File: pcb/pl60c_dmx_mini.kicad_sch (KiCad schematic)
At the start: 35 parts, among them J1 USB-C 16P, J2 XLR-5 female (DMX OUT), Q1 S8050, SW2 BOOT, SW3 USER, U1 ESP32-S3-MINI-1-N8, U2 AP2112K-3.3, U3 SP3485EN, U4 USBLC6-2SC6

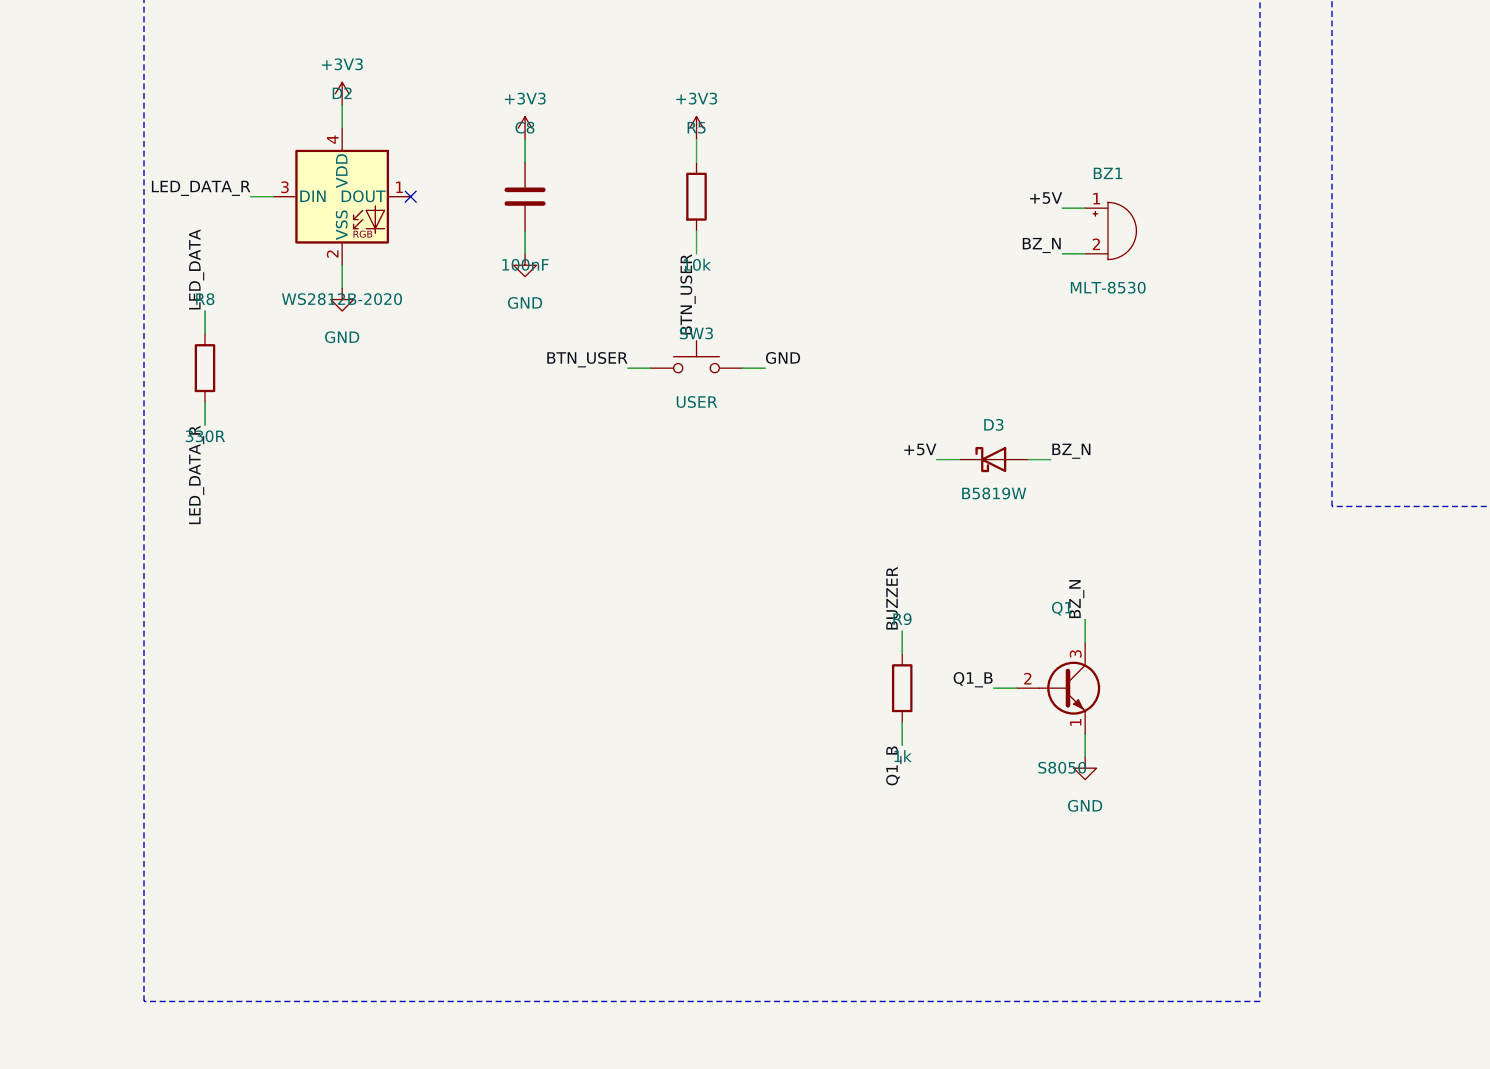
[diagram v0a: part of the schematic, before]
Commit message: auto: 2026-09-02 14:14:01
Co-Authored-By: Claude Fable 5.1 <noreply@anthropic.com>
Claude-Session: https://claude.ai/code/session_01WsrVZb94LwbHVAmBvsSTfn
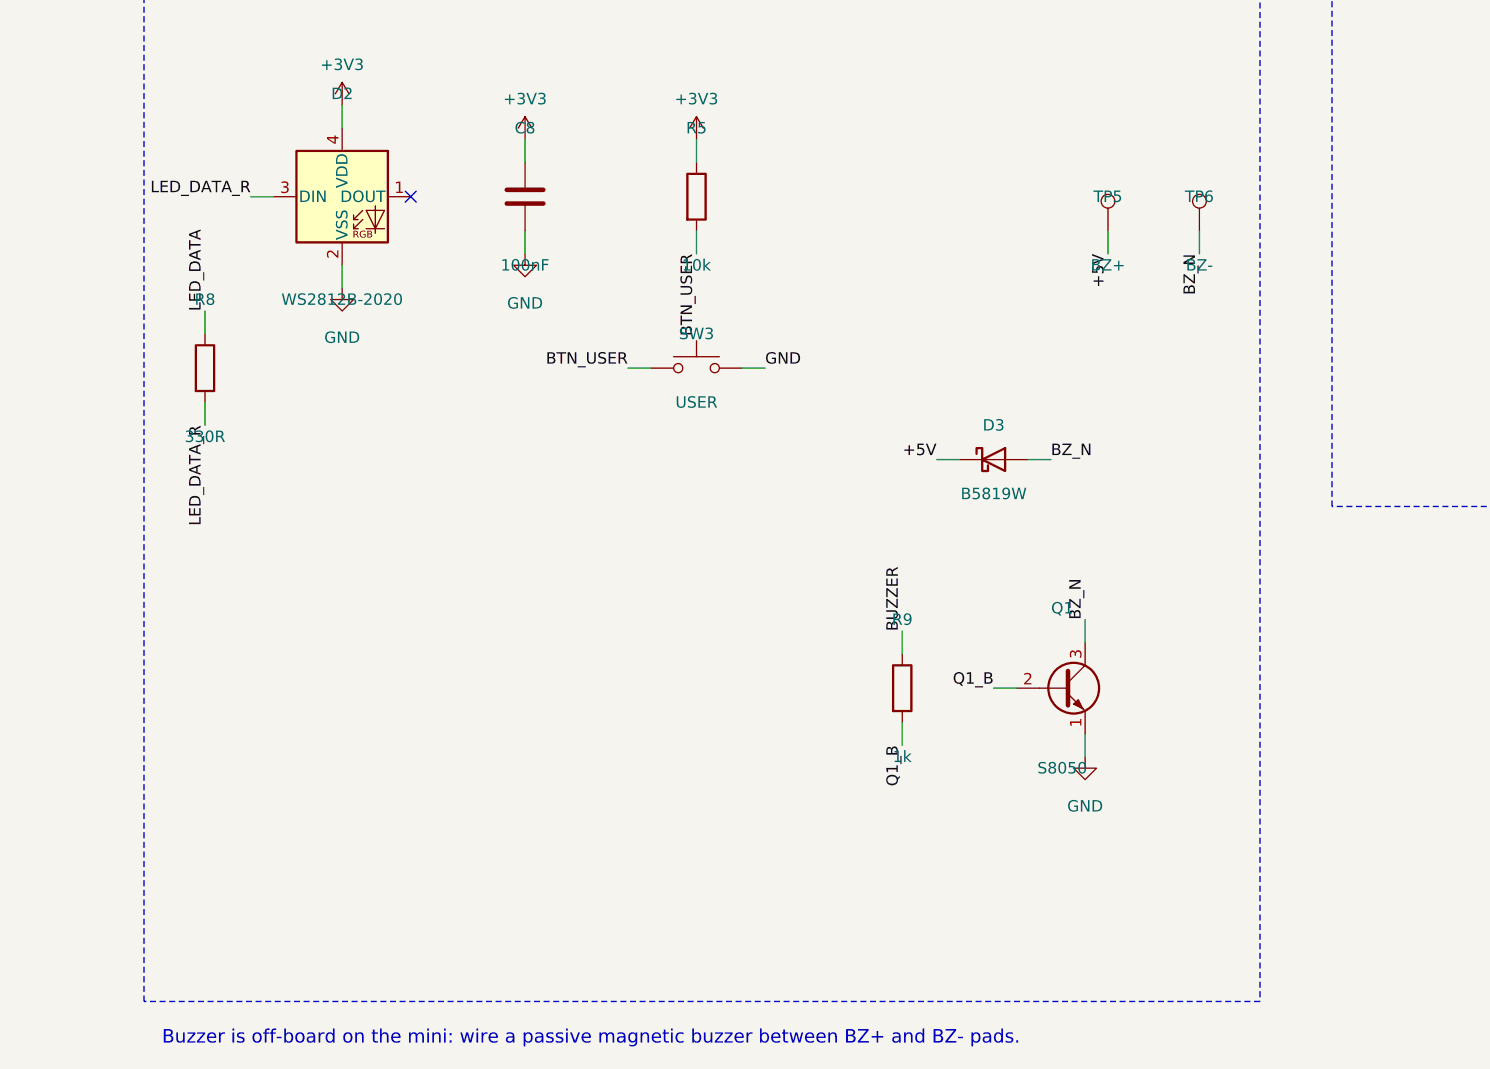
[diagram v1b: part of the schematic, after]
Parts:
- removed BZ1: MLT-8530, Buzzer_Beeper:MagneticBuzzer_CUI_CMT-8504-100-SMT, symbol Device:Buzzer
- added TP5: BZ+, TestPoint:TestPoint_Pad_1.5x1.5mm, symbol Connector:TestPoint
- added TP6: BZ-, TestPoint:TestPoint_Pad_1.5x1.5mm, symbol Connector:TestPoint
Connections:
- net +5V: now also TP5.1
- net BZ_N: now also TP6.1
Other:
- note added: "Buzzer is off-board on the mini: wire a passive magnetic buzzer between BZ+ and BZ- pads."
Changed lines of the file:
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@@
 	)
 	(symbol
-		(lib_id "Device:Buzzer")
+		(lib_id "Connector:TestPoint")
 		(at 245.11 199.39 0)
 		(unit 1)
@@
 		(on_board yes)
 		(dnp no)
-		(property "Reference" "BZ1"
-			(at 245.11 193.04 0)
-			(effects
-				(font
-					(size 1.27 1.27)
-				)
-			)
-		)
-		(property "Value" "MLT-8530"
-			(at 245.11 205.74 0)
-			(effects
-				(font
-					(size 1.27 1.27)
-				)
-			)
-		)
-		(property "Footprint" "Buzzer_Beeper:MagneticBuzzer_CUI_CMT-8504-100-SMT"
+		(property "Reference" "TP5"
+			(at 245.11 195.58 0)
+			(effects
+				(font
+					(size 1.27 1.27)
+				)
+			)
+		)
+		(property "Value" "BZ+"
+			(at 245.11 203.2 0)
+			(effects
+				(font
+					(size 1.27 1.27)
+				)
+			)
+		)
+		(property "Footprint" "TestPoint:TestPoint_Pad_1.5x1.5mm"
 			(at 245.11 199.39 0)
 			(effects
@@
 			)
 		)
-		(property "Description" "Magnetic buzzer 8.5x8.5 mm SMD, passive, 16 ohm"
+		(property "Description" "External buzzer pad (+5V)"
 			(at 245.11 199.39 0)
 			(effects
@@
 			)
 		)
-		(property "LCSC" "C94599"
+		(property "LCSC" ""
 			(at 245.11 199.39 0)
 			(effects
@@
 			)
 		)
-		(property "MPN" "MLT-8530"
-			(at 245.11 199.39 0)
-			(effects
-				(font
-					(size 1.27 1.27)
-				)
-				(hide yes)
-			)
-		)
-		(pin "1"
-		)
-		(pin "2"
-		)
-		(instances
-			(project "pl60c_dmx_mini"
-				(path "/e63f84e3-7254-5f79-8caa-7afae8cc707c"
-					(reference "BZ1")
+		(pin "1"
+		)
+		(instances
+			(project "pl60c_dmx_mini"
+				(path "/e63f84e3-7254-5f79-8caa-7afae8cc707c"
+					(reference "TP5")
 					(unit 1)
 				)
@@
 	(wire
 		(pts
-			(xy 242.57 196.85)
-			(xy 240.03 196.85)
+			(xy 245.11 199.39)
+			(xy 245.11 201.93)
 		)
 		(stroke
@@
 	)
 	(label "+5V"
-		(at 240.03 196.85 180)
+		(at 245.11 201.93 270)
 		(fields_autoplaced yes)
 		(effects
@@
 			)
 			(justify right bottom)
+		)
+	)
+	(symbol
+		(lib_id "Connector:TestPoint")
+		(at 255.27 199.39 0)
+		(unit 1)
+		(exclude_from_sim no)
+		(in_bom yes)
+		(on_board yes)
+		(dnp no)
+		(property "Reference" "TP6"
+			(at 255.27 195.58 0)
+			(effects
+				(font
+					(size 1.27 1.27)
+				)
+			)
+		)
+		(property "Value" "BZ-"
+			(at 255.27 203.2 0)
+			(effects
+				(font
+					(size 1.27 1.27)
+				)
+			)
+		)
+		(property "Footprint" "TestPoint:TestPoint_Pad_1.5x1.5mm"
+			(at 255.27 199.39 0)
+			(effects
+				(font
+					(size 1.27 1.27)
+				)
+				(hide yes)
+			)
+		)
+		(property "Datasheet" "~"
+			(at 255.27 199.39 0)
+			(effects
+				(font
+					(size 1.27 1.27)
+				)
+				(hide yes)
+			)
+		)
+		(property "Description" "External buzzer pad (driver collector)"
+			(at 255.27 199.39 0)
+			(effects
+				(font
+					(size 1.27 1.27)
+				)
+				(hide yes)
+			)
+		)
+		(property "LCSC" ""
+			(at 255.27 199.39 0)
+			(effects
+				(font
+					(size 1.27 1.27)
+				)
+				(hide yes)
+			)
+		)
+		(pin "1"
+		)
+		(instances
+			(project "pl60c_dmx_mini"
+				(path "/e63f84e3-7254-5f79-8caa-7afae8cc707c"
+					(reference "TP6")
+					(unit 1)
+				)
+			)
 		)
 	)
 	(wire
 		(pts
-			(xy 242.57 201.93)
-			(xy 240.03 201.93)
+			(xy 255.27 199.39)
+			(xy 255.27 201.93)
 		)
 		(stroke
@@
 	)
 	(label "BZ_N"
-		(at 240.03 201.93 180)
+		(at 255.27 201.93 270)
 		(fields_autoplaced yes)
 		(effects
@@
 		(effects
 			(font
+				(size 1.5 1.5)
+			)
+			(justify left bottom)
+		)
+	)
+	(text "Buzzer is off-board on the mini: wire a passive magnetic buzzer between BZ+ and BZ- pads."
+		(exclude_from_sim no)
+		(at 140 290 0)
+		(effects
+			(font
